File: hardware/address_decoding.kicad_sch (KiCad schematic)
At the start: 9 parts, among them U2 74HC30, U3 74AHC00, U4 74AHC32, U5 74AHC138

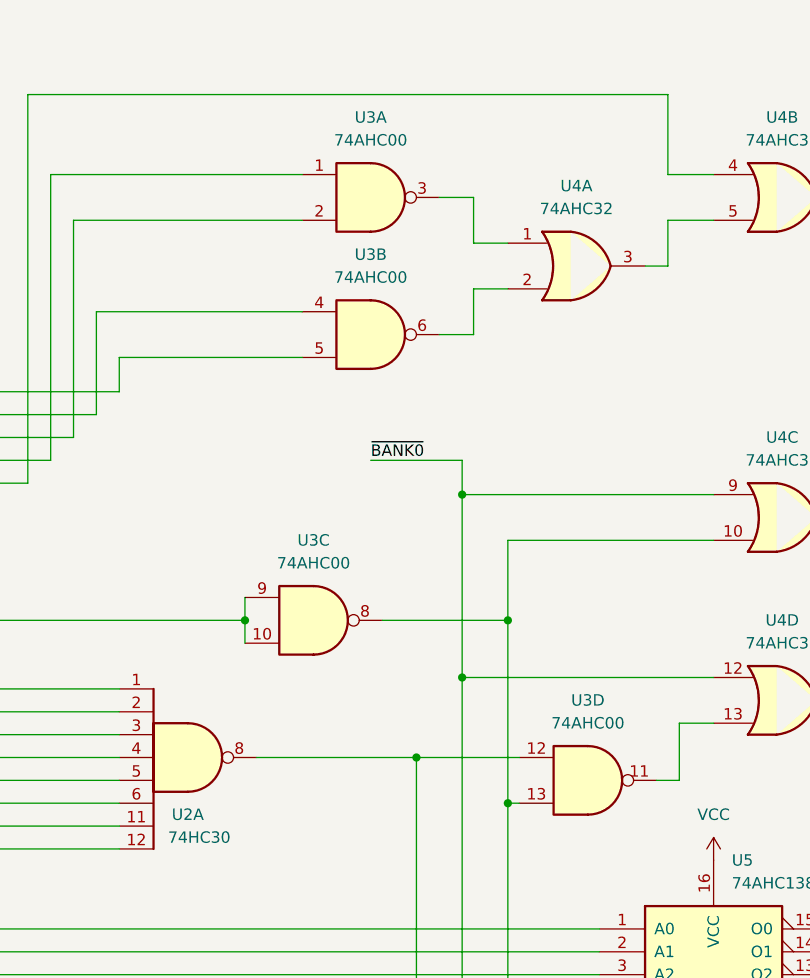
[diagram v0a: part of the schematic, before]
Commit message: Kicad 7
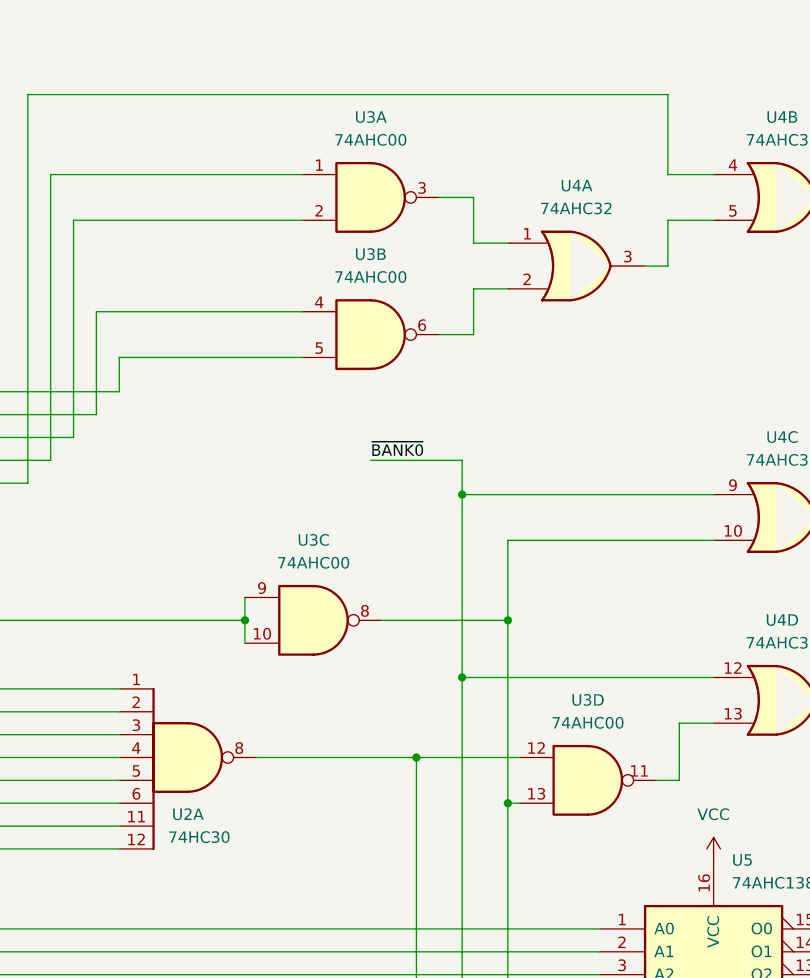
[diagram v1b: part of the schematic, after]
